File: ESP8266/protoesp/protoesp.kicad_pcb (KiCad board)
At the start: 2 copper layers, 97.5 x 97.5 mm, 147 parts, among them CN1 EPINS_TOP, CN10 USB_CURSED, CN11 CH_SPI, CN12 CH_I2C, CN13 CH341_PROG, CN14 CH_PROG, CN2 EPINS_BOTTOM, CN20 BATT, CN3 ESP_PROG, CN30 BUTTON_CONN, CN31 LDR_CONN, CN32 RGB_CONN, CN33 595_CONN, CN34 E_SPI, CN35 E_I2C, CN36 DRV_CONN, CN47 595_OUTS, J1 0R, J11 0R, J17 0R, J19 0R, J22 0R, J7 0R, J8 0R, J9 0R, Q1 BC817, Q2 CJ2305, SW1 RST, SW2 BUTTON, U1 CH341, U2 AP1117-33, U3 LTH7R, U4 74HC595, U5 AP2112K-3.3, U6 ESP32-WROOM-32, Y1 12MHz

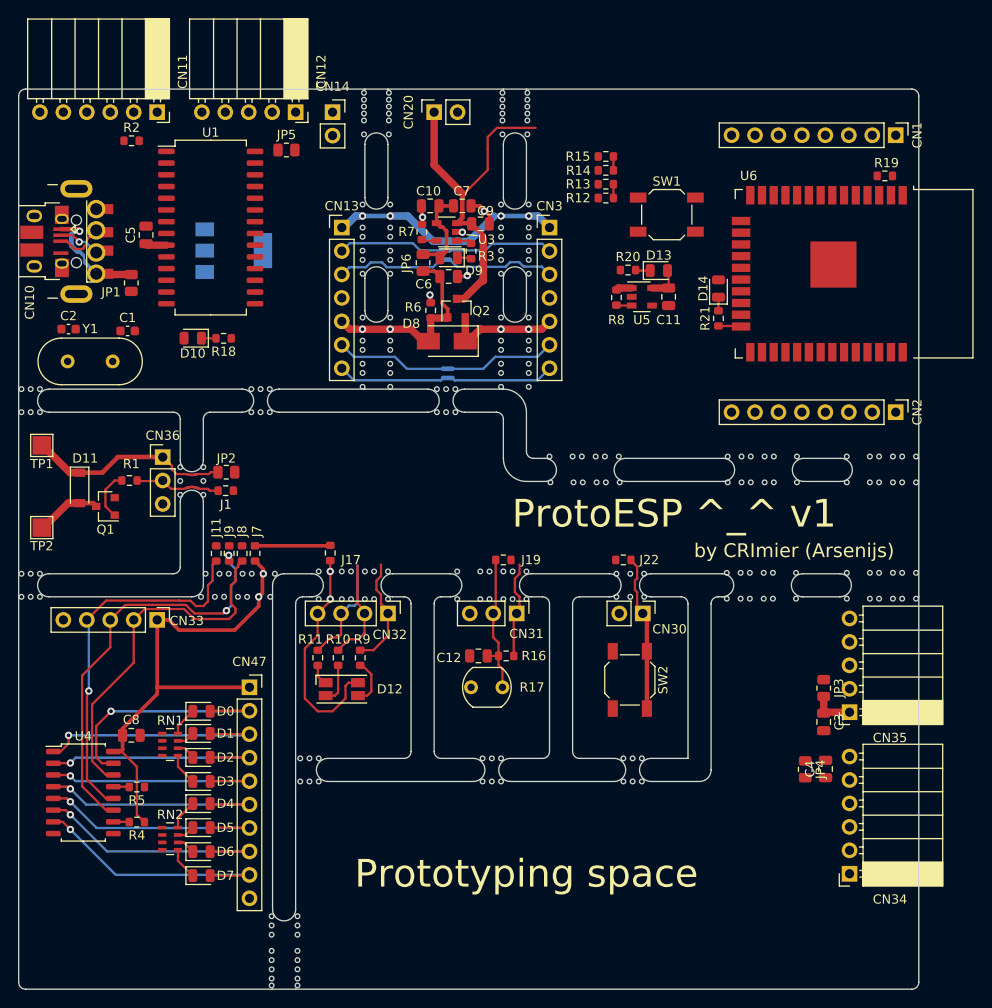
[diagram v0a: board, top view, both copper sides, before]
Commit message: ProtoESP work day 7
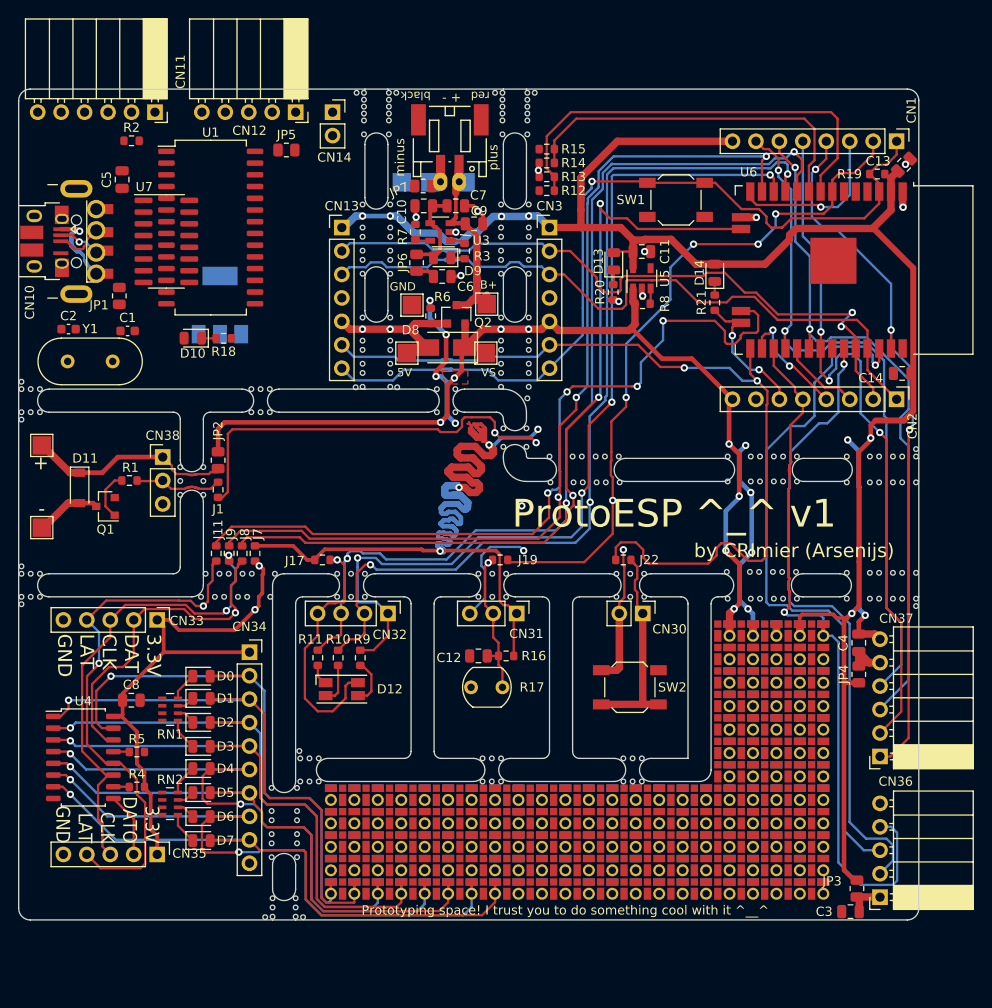
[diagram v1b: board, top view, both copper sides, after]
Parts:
- removed CN47: 595_OUTS, Connector_PinSocket_2.54mm:PinSocket_1x10_P2.54mm_Vertical
- removed the REF** at (134.2, 102.4)
- removed the REF** at (134.2, 105.2)
- removed the REF** at (95.3, 85.0)
- removed the REF** at (95.3, 82.5)
- removed the REF** at (97.5, 102.2)
- removed the REF** at (97.5, 105.2)
- removed the REF** at (82.5, 105.2)
- removed the REF** at (82.5, 102.2)
- removed the REF** at (77.4, 139.6)
- removed the REF** at (80.2, 139.6)
- added C13: 1uF, Capacitor_SMD:C_0805_2012Metric, F.Cu at (145.9, 58.2)
- added C14: 100nF, Capacitor_SMD:C_0805_2012Metric, F.Cu at (145.7, 80.8)
- added CN34: 595_OUTS, Connector_PinSocket_2.54mm:PinSocket_1x10_P2.54mm_Vertical, F.Cu at (75.0, 111.0)
- added CN36: E_I2C, Connector_PinSocket_2.54mm:PinSocket_1x05_P2.54mm_Horizontal, F.Cu at (143.3, 137.5)
- added JP7: 0R, Resistor_SMD:R_0805_2012Metric, F.Cu at (93.8, 60.5)
- added P1: PROTO_SPACE, protoesp:PROTO_THT_SMD_FULL, F.Cu at (127.0, 127.0)
- added REF**: mouse_2sig_3mm, protoesp:mouse_2mm_1sig, F.Cu at (105.0, 88.8)
- added REF**: mouse_2sig_3mm, protoesp:mouse_single, F.Cu at (76.7, 139.7)
- added REF**: mouse_2sig_3mm, protoesp:mouse_single, F.Cu at (80.8, 139.7)
- added REF**: mouse_2sig_3mm, protoesp:mouse_single, F.Cu at (147.2, 106.0)
- added REF**: mouse_2sig_3mm, protoesp:mouse_single, F.Cu at (147.2, 89.0)
- added REF**: mouse_2sig_3mm, protoesp:mouse_single, F.Cu at (86.6, 50.4)
- added REF**: mouse_2sig_3mm, protoesp:mouse_single, F.Cu at (90.9, 50.4)
- added REF**: mouse_2sig_3mm, protoesp:mouse_single, F.Cu at (101.6, 50.4)
- added REF**: mouse_2sig_3mm, protoesp:mouse_single, F.Cu at (105.9, 50.4)
- added REF**: mouse_2sig_3mm, protoesp:mouse_single, F.Cu at (91.0, 82.3)
- added REF**: mouse_2sig_3mm, protoesp:mouse_single, F.Cu at (86.5, 82.3)
- added REF**: mouse_2sig_3mm, protoesp:mouse_2mm_1sig, F.Cu at (102.5, 88.8)
- added REF**: mouse_2sig_3mm, protoesp:mouse_single, F.Cu at (50.3, 81.7)
- added REF**: mouse_2sig_3mm, protoesp:mouse_single, F.Cu at (50.3, 85.8)
- added REF**: mouse_2sig_3mm, protoesp:mouse_single, F.Cu at (50.3, 101.7)
- added REF**: mouse_2sig_3mm, protoesp:mouse_single, F.Cu at (50.3, 105.8)
- added REF**: mouse_2sig_3mm, protoesp:mouse_single, F.Cu at (105.1, 83.5)
- added REF**: mouse_1power_2sig_7.5mm, protoesp:mouse_1power_2sig_7.5mm, F.Cu at (77.4, 125.7)
- added REF**: mouse_1power_2sig_7.5mm, protoesp:mouse_1power_2sig_7.5mm, F.Cu at (80.2, 125.7)
- added REF**: mouse_2sig_3mm, protoesp:mouse_2mm, F.Cu at (77.5, 139.7)
- added REF**: mouse_2sig_3mm, protoesp:mouse_2mm, F.Cu at (80.0, 139.7)
- added REF**: mouse_2sig_3mm, protoesp:mouse_2mm_1sig, F.Cu at (95.3, 85.0)
- added REF**: mouse_1power_2sig_7.5mm, protoesp:mouse_1power_2sig_7.5mm, F.Cu at (126.7, 102.3)
- added REF**: mouse_2sig_3mm, protoesp:mouse_2mm_1sig, F.Cu at (95.3, 82.5)
- added REF**: mouse_1power_2sig_7.5mm, protoesp:mouse_1power_2sig_7.5mm, F.Cu at (126.8, 105.2)
- added REF**: mouse_2sig_3mm, protoesp:mouse_2sig_3mm, F.Cu at (84.5, 102.5)
- added REF**: mouse_2sig_3mm, protoesp:mouse_2sig_3mm, F.Cu at (84.5, 105.0)
- added REF**: mouse_2sig_3mm, protoesp:mouse_2sig_3mm, F.Cu at (99.8, 102.5)
- added REF**: mouse_2sig_3mm, protoesp:mouse_2sig_3mm, F.Cu at (99.8, 105.0)
- added REF**: mouse_2sig_3mm, protoesp:mouse_single, F.Cu at (80.4, 121.7)
- added TP3: B+, TestPoint:TestPoint_Pad_2.0x2.0mm, F.Cu at (100.7, 73.3)
- added TP4: 5V, TestPoint:TestPoint_Pad_2.0x2.0mm, F.Cu at (92.0, 78.6)
- added TP5: GND, TestPoint:TestPoint_Pad_2.0x2.0mm, F.Cu at (92.6, 73.4)
- added TP6: VS, TestPoint:TestPoint_Pad_2.0x2.0mm, F.Cu at (100.6, 78.6)
- added TP7: B+, TestPoint:TestPoint_Pad_2.0x2.0mm, B.Cu at (94.6, 60.1)
- added TP8: B+, TestPoint:TestPoint_Pad_2.0x2.0mm, B.Cu at (98.4, 60.1)
- added TP9: GND, TestPoint:TestPoint_Pad_2.0x2.0mm, B.Cu at (91.5, 60.1)
- added U7: CH340G, Package_SO:SOIC-16_3.9x9.9mm_P1.27mm, F.Cu at (66.0, 66.5)
- CN20: footprint Connector_PinSocket_2.54mm:PinSocket_1x02_P2.54mm_Vertical -> protoesp:JST_PH_S2B-PH-SM4-TB_02x2.00mm_Angled
- CN35: value E_I2C -> 595CHAIN_CONN; footprint Connector_PinSocket_2.54mm:PinSocket_1x05_P2.54mm_Horizontal -> Connector_PinHeader_2.54mm:PinHeader_1x05_P2.54mm_Vertical
- moved CN35 76.6 mm to (65.0, 132.9), turned to 270 degrees
- moved JP3 22.0 mm to (140.8, 136.6)
- moved C3 20.8 mm to (140.1, 139.1), turned to 180 degrees
- moved C4 14.1 mm to (141.0, 110.0)
- moved CN37 13.1 mm to (143.3, 122.3)
- moved JP4 11.8 mm to (141.0, 113.4), turned to 90 degrees
- moved REF** 7.50 mm to (126.8, 92.5), turned to 0 degrees
- moved REF** 7.50 mm to (126.8, 89.8), turned to 0 degrees
- moved C5 6.54 mm to (61.2, 59.8)
- moved R12 6.45 mm to (107.2, 61.0)
- moved R13 6.45 mm to (107.2, 59.5)
- moved R14 6.45 mm to (107.2, 58.0)
- moved R15 6.45 mm to (107.2, 56.5)
- moved U2 6.09 mm to (71.8, 73.4), turned to 90 degrees
- moved C11 5.69 mm to (117.5, 67.6), turned to 0 degrees
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- renumbered CN34 to CN37, CN36 to CN38
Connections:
- net Net-(CN47-Pad2) renamed /5D0
- net Net-(CN47-Pad3) renamed /5D1
- net Net-(CN47-Pad4) renamed /5D2
- net Net-(CN47-Pad5) renamed /5D3
- net Net-(CN47-Pad6) renamed /5D4
- net Net-(CN47-Pad7) renamed /5D5
- net Net-(CN47-Pad8) renamed /5D6
- net Net-(CN47-Pad9) renamed /5D7
- CN20 pad 2: GND -> -BATT
- CN35 pad 1: Net-(C3-Pad1) -> VCC_595
- CN35 pad 2: E_SDA -> 595_DAT_O
- CN35 pad 3: E_SCL -> 595_CLK_J
- CN35 pad 4: E_INT -> 595_LAT_J
- U4 pad 9: Net-(U4-Pad9) -> 595_DAT_O
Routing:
- net +3V3: track 48.3 -> 301.9 mm, vias 4 -> 10
- net GND: track 8.92 -> 111.8 mm, vias 5 -> 23
- net 595_CLK: track 0.00 -> 100.3 mm, vias 0 -> 3
- net +VSW: track 14.3 -> 109.2 mm, vias 2 -> 8
- net LED_RED: track 11.8 -> 104.2 mm, vias 0 -> 3
- net 595_DAT: track 0.00 -> 91.0 mm, vias 0 -> 3
- net LED_GREEN: track 11.4 -> 100.6 mm, vias 0 -> 3
- net LED_BLUE: track 12.1 -> 99.4 mm, vias 0 -> 4
- net 595_LAT: track 0.00 -> 85.8 mm, vias 0 -> 4
- net E_INT: track 0.00 -> 79.3 mm, vias 0 -> 1
- net E_MOSI: track 0.00 -> 76.9 mm, vias 0 -> 3
- net E_MISO: track 0.00 -> 76.1 mm, vias 0 -> 3
- net E_SCL: track 0.00 -> 75.6 mm, vias 0 -> 1
- net E_SCK: track 0.00 -> 75.3 mm, vias 0 -> 2
- net E_CS: track 0.00 -> 75.1 mm, vias 0 -> 2
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- added copper zone on F.Cu, net +VSW
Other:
- board size 97.5 x 97.5 mm -> 97.5 x 90 mm
- board text added: "- +"
- board text added: "3.3V D0 D1 D2 D3 D4 D5 D6 D7 GND"
- board text added: "3.3V DAT CLK LAT GND"
- board text added: "3.3V DATO CLK LAT GND"
- board text added: "3.3V DAT_O CLK LAT GND"
- board text added: "GND D+ D- 5V"
- board text added: "Power"
- board text added: "Prototyping space! I trust you to do something cool with it ^__^"
- board text added: "VSW GND"
- board text added: "black"
- board text added: "minus"
- board text added: "plus"
- board text added: "red"
- board text removed: "Prototyping space"
